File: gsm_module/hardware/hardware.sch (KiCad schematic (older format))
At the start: 65 parts, among them J1 Screw_Terminal_01x04, J10 Conn_01x02_Male, J11 Conn_01x02_Male, J12 Conn_01x02_Male, J13 Conn_01x02_Male, J2 78646-3001, J4 Programming interface, J5 SWD Debugging Interface, J6 Conn_01x02_Male, J7 Conn_01x02_Male, J8 Conn_01x02_Male, J9 Conn_01x02_Male, U1 XL1509-ADJ, U10 XL1509-ADJ, U2 AMS1117-3.3, U3 MCP2515-xSO, U4 STM32F030F4Px, U5 MCP2551-I-SN, U6 SIM868, Y1 8mhz

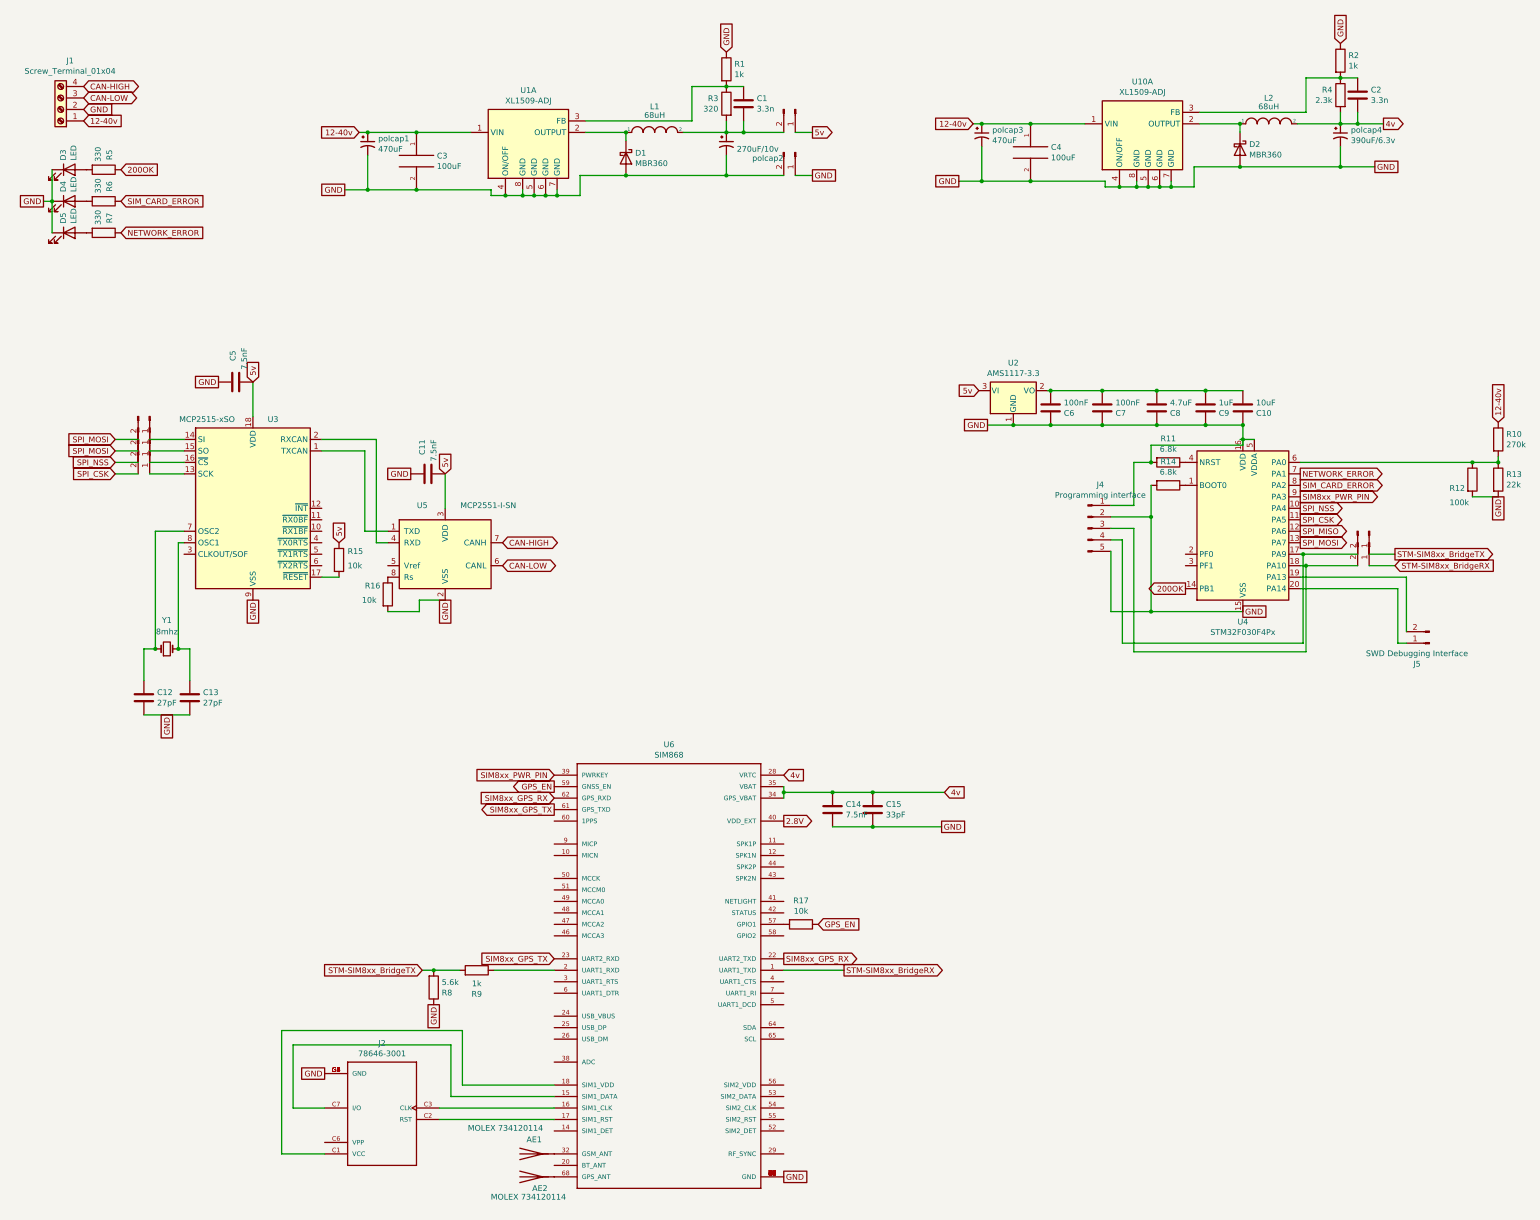
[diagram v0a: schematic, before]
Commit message: rev .5 PCB motherfucker (we-ho)
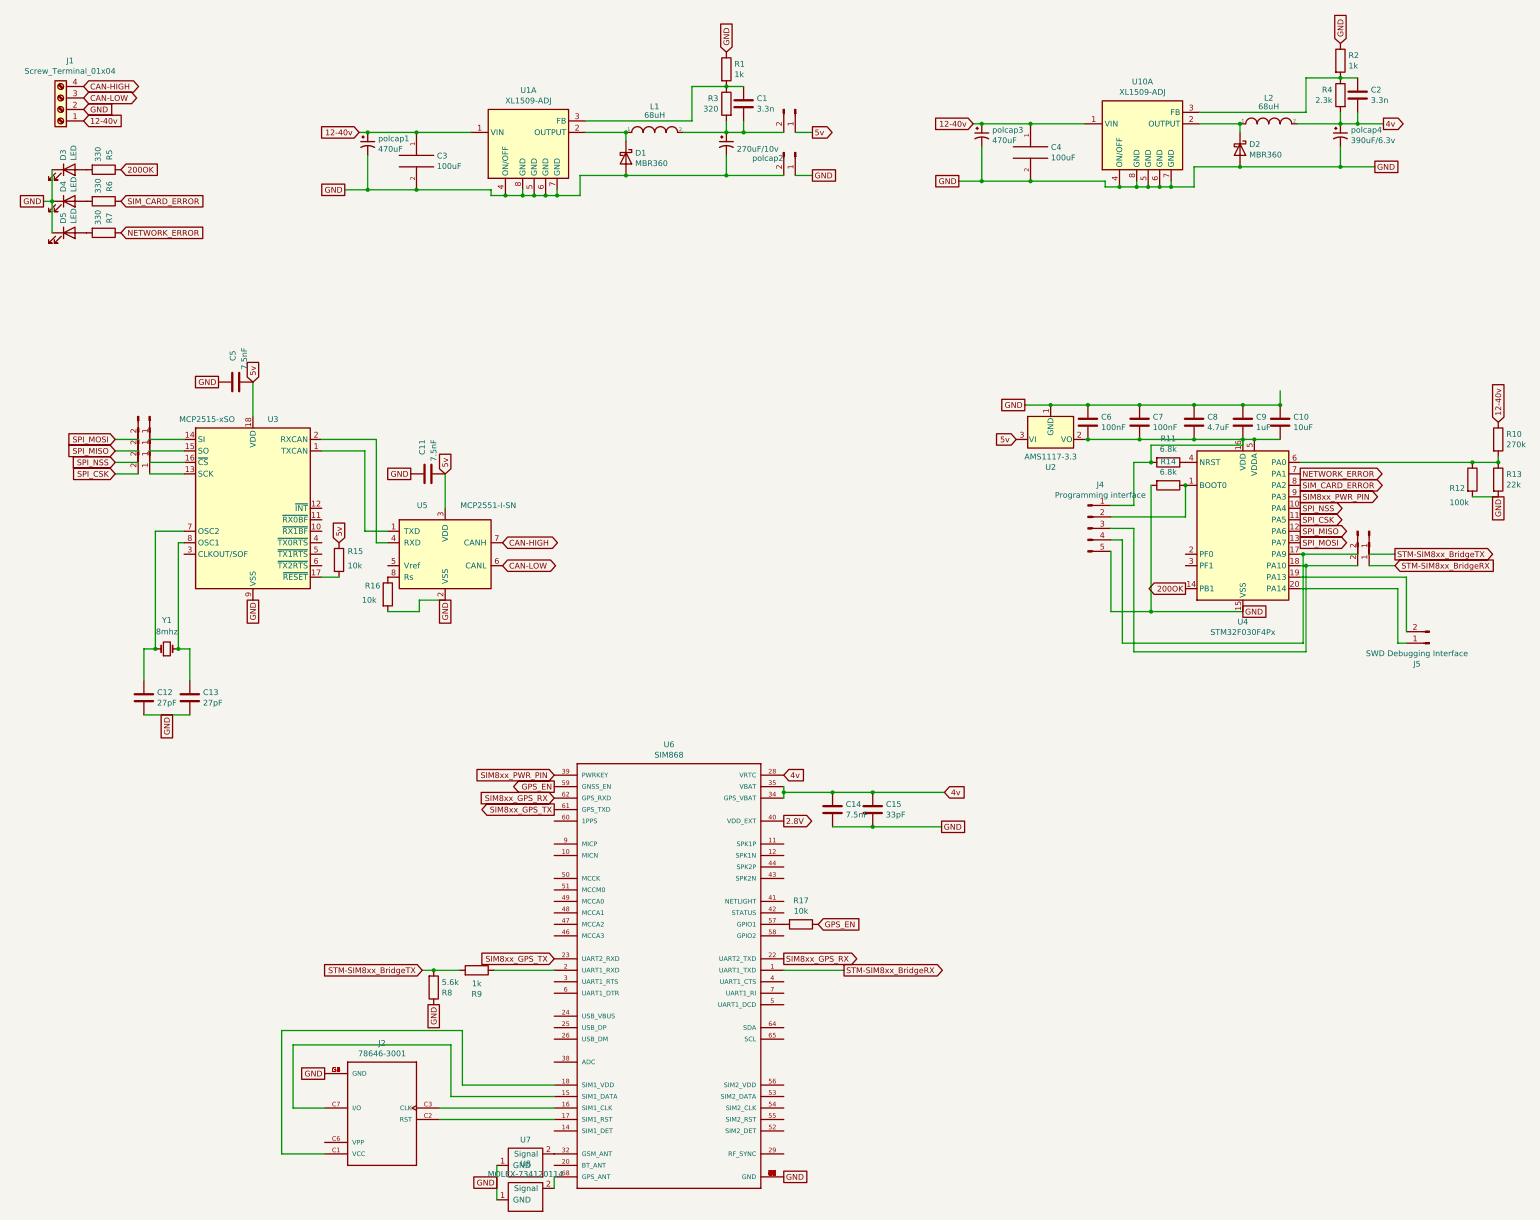
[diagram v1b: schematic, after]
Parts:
- removed AE1, AE2: MOLEX 734120114, its_app:KH-IPEX4-2020, symbol Device:Antenna
- added U7, U8: MOLEX-734120114, its_app:KH-IPEX4-2020, symbol SIM868:MOLEX-734120114
- J10, J11, J12, J13, J5, J6, J7, J8, J9: footprint Connector_PinHeader_1.00mm:PinHeader_1x02_P1.00mm_Vertical -> Connector_PinHeader_2.54mm:PinHeader_1x02_P2.54mm_Vertical
- J4: footprint Connector_PinHeader_1.00mm:PinHeader_1x05_P1.00mm_Vertical -> Connector_PinHeader_2.54mm:PinHeader_1x05_P2.54mm_Vertical
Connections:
- net GND: now also U7.1 (GND), U8.1 (GND); no longer J4.1 (Pin_1), J4.2 (Pin_2), R11.2, U4.16 (VDD), U4.5 (VDDA)
- net SPI_MISO: now also J9.2 (Pin_2)
- net SPI_MOSI: no longer J9.2 (Pin_2)
- net at R14.1, U4.1 (BOOT0): now also J4.2 (Pin_2)
- net at C10.2, C6.2, C7.2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: now also J4.1 (Pin_1), R11.2, U4.16 (VDD), U4.5 (VDDA)
- net at U6.32 (GSM_ANT): now also U7.2 (Signal)
- net at U6.68 (GPS_ANT): now also U8.2 (Signal)
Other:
- moved on the sheet: C10, C6, C7, C8, C9, U2
